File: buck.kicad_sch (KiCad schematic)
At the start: 23 parts, among them IC2 LV2862YDDCR, IC2 RT6285GSP

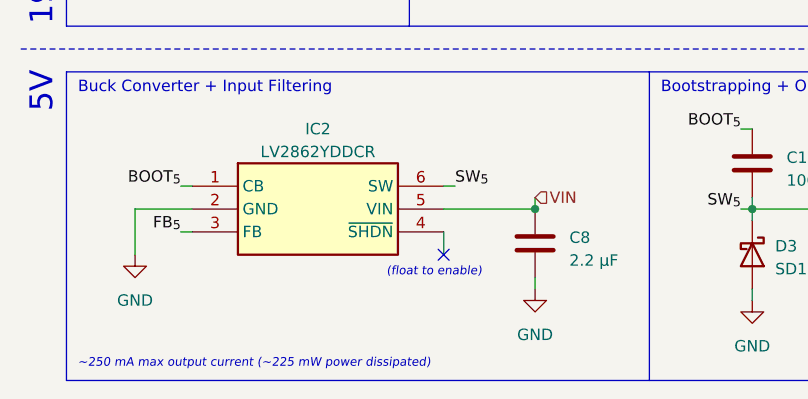
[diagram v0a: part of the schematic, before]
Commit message: Create new STEP files
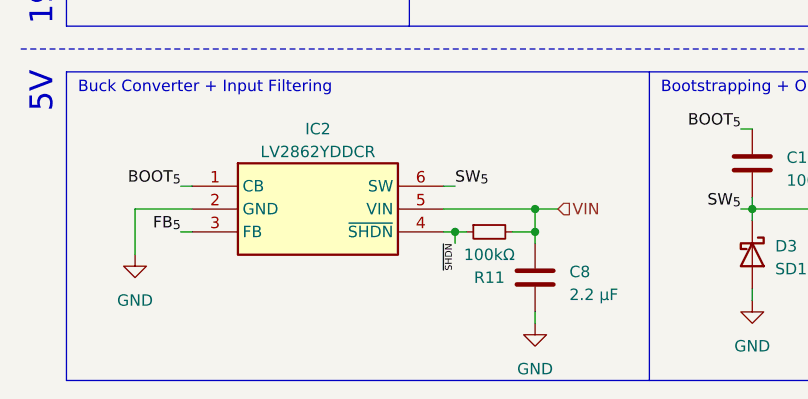
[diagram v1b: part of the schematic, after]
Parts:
- added R11: 100kΩ, Resistor_SMD:R_0603_1608Metric_Pad0.98x0.95mm_HandSolder, symbol Device:R_Small
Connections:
- net VIN: now also R11.2
- net ~{SHDN}: now reaches IC2.4 (~{SHDN})
- net ~{SHDN}: now also R11.1
- no-connect marks 4 -> 3
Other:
- note removed: "(float to enable)"
- note removed: "~250 mA max output current (~225 mW power dissipated)"
- moved on the sheet: C8
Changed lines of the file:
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@@
     (company "UT RoboMasters")
   )
+  (junction (at 91.44 133.35) (diameter 0) (color 0 0 0 0)
+  )
   (junction (at 100.33 130.81) (diameter 0) (color 0 0 0 0)
   )
@@
   (junction (at 135.89 57.15) (diameter 0) (color 0 0 0 0)
   )
+  (junction (at 100.33 133.35) (diameter 0) (color 0 0 0 0)
+  )
   (junction (at 97.79 60.96) (diameter 0) (color 0 0 0 0)
   )
@@
   )
   (no_connect (at 170.18 69.85))
-  (no_connect (at 90.17 135.89))
   (no_connect (at 200.66 74.93))
   (no_connect (at 170.18 72.39))
@@
     (stroke (width 0) (type default))
   )
-  (wire (pts (xy 90.17 135.89) (xy 90.17 133.35))
+  (wire (pts (xy 102.87 130.81) (xy 100.33 130.81))
     (stroke (width 0) (type default))
   )
@@
   )
   (wire (pts (xy 124.46 129.54) (xy 124.46 130.81))
+    (stroke (width 0) (type default))
+  )
+  (wire (pts (xy 91.44 134.62) (xy 91.44 133.35))
     (stroke (width 0) (type default))
   )
@@
     (stroke (width 0) (type dash))
   )
-  (wire (pts (xy 100.33 138.43) (xy 100.33 139.7))
+  (wire (pts (xy 100.33 142.24) (xy 100.33 143.51))
     (stroke (width 0) (type default))
   )
@@
     (stroke (width 0) (type default))
   )
+  (wire (pts (xy 97.79 133.35) (xy 100.33 133.35))
+    (stroke (width 0) (type default))
+  )
+  (wire (pts (xy 100.33 133.35) (xy 100.33 130.81))
+    (stroke (width 0) (type default))
+  )
   (polyline (pts (xy 86.36 78.74) (xy 156.21 78.74))
     (stroke (width 0) (type default))
   )
+  (wire (pts (xy 90.17 133.35) (xy 91.44 133.35))
+    (stroke (width 0) (type default))
+  )
   (wire (pts (xy 133.35 97.79) (xy 133.35 99.06))
     (stroke (width 0) (type default))
@@
     (stroke (width 0) (type default))
   )
-  (wire (pts (xy 100.33 129.54) (xy 100.33 130.81))
+  (wire (pts (xy 100.33 134.62) (xy 100.33 133.35))
     (stroke (width 0) (type default))
   )
@@
     (stroke (width 0) (type default))
   )
+  (wire (pts (xy 91.44 133.35) (xy 92.71 133.35))
+    (stroke (width 0) (type default))
+  )
   (wire (pts (xy 123.19 121.92) (xy 124.46 121.92))
     (stroke (width 0) (type default))
@@
   (wire (pts (xy 144.78 130.81) (xy 146.05 130.81))
     (stroke (width 0) (type default))
-  )
-  (text "(float to enable)" (at 83.82 138.43 0)
-    (effects (font (size 0.96 0.96) italic) (justify left bottom))
   )
   (text "Buck converter controller" (at 158.75 49.53 0)
@@
     (effects (font (size 1.27 1.27)) (justify left bottom))
   )
-  (text "~250 mA max output current (~225 mW power dissipated)"
-    (at 49.53 148.59 0)
-    (effects (font (size 0.96 0.96) italic) (justify left bottom))
-  )
   (label "BOOT_{5}" (at 123.19 121.92 180) (fields_autoplaced)
     (effects (font (size 1.27 1.27)) (justify right bottom))
   )
+  (label "~{SHDN}" (at 91.44 134.62 270) (fields_autoplaced)
+    (effects (font (size 0.762 0.762)) (justify right bottom))
+  )
   (label "BOOT_{19}" (at 168.91 67.31 180) (fields_autoplaced)
     (effects (font (size 1.27 1.27)) (justify right bottom))
@@
     (effects (font (size 1.27 1.27)) (justify left))
   )
-  (hierarchical_label "VIN" (shape input) (at 100.33 129.54 0) (fields_autoplaced)
+  (hierarchical_label "VIN" (shape input) (at 102.87 130.81 0) (fields_autoplaced)
     (effects (font (size 1.27 1.27)) (justify left))
   )
@@
     )
   )
-  (symbol (lib_id "Device:C") (at 100.33 134.62 0) (unit 1)
+  (symbol (lib_id "Device:C") (at 100.33 138.43 0) (unit 1)
     (in_bom yes) (on_board yes) (dnp no)
-    (property "Reference" "C8" (at 104.14 133.985 0)
-      (effects (font (size 1.27 1.27)) (justify left))
-    )
-    (property "Value" "2.2 μF" (at 104.14 136.525 0)
-      (effects (font (size 1.27 1.27)) (justify left))
-    )
-    (property "Footprint" "Capacitor_SMD:C_0603_1608Metric_Pad1.08x0.95mm_HandSolder" (at 101.2952 138.43 0)
-      (effects (font (size 1.27 1.27)) hide)
-    )
-    (property "Datasheet" "https://www.mouser.com/datasheet/2/585/MLCC-1837944.pdf" (at 100.33 134.62 0)
+    (property "Reference" "C8" (at 104.14 137.795 0)
+      (effects (font (size 1.27 1.27)) (justify left))
+    )
+    (property "Value" "2.2 μF" (at 104.14 140.335 0)
+      (effects (font (size 1.27 1.27)) (justify left))
+    )
+    (property "Footprint" "Capacitor_SMD:C_0603_1608Metric_Pad1.08x0.95mm_HandSolder" (at 101.2952 142.24 0)
+      (effects (font (size 1.27 1.27)) hide)
+    )
+    (property "Datasheet" "https://www.mouser.com/datasheet/2/585/MLCC-1837944.pdf" (at 100.33 138.43 0)
       (effects (font (size 1.27 1.27)) hide)
     )
@@
     )
   )
-  (symbol (lib_id "power:GND") (at 100.33 139.7 0) (unit 1)
-    (in_bom yes) (on_board yes) (dnp no) (fields_autoplaced)
-    (property "Reference" "#PWR035" (at 100.33 146.05 0)
-      (effects (font (size 1.27 1.27)) hide)
-    )
-    (property "Value" "GND" (at 100.33 144.78 0)
-      (effects (font (size 1.27 1.27)))
-    )
-    (property "Footprint" "" (at 100.33 139.7 0)
-      (effects (font (size 1.27 1.27)) hide)
-    )
-    (property "Datasheet" "" (at 100.33 139.7 0)
-      (effects (font (size 1.27 1.27)) hide)
-    )
+  (symbol (lib_id "Device:R_Small") (at 95.25 133.35 90) (mirror x) (unit 1)
+    (in_bom yes) (on_board yes) (dnp no)
+    (property "Reference" "R11" (at 95.25 138.43 90)
+      (effects (font (size 1.27 1.27)))
+    )
+    (property "Value" "100kΩ" (at 95.25 135.89 90)
+      (effects (font (size 1.27 1.27)))
+    )
+    (property "Footprint" "Resistor_SMD:R_0603_1608Metric_Pad0.98x0.95mm_HandSolder" (at 95.25 133.35 0)
+      (effects (font (size 1.27 1.27)) hide)
+    )
+    (property "Datasheet" "~" (at 95.25 133.35 0)
+      (effects (font (size 1.27 1.27)) hide)
+    )
+    (pin "1")
+    (pin "2")
+    (instances
+      (project "Chassis"
+        (path "/d5f28ba3-2393-441a-9a3a-5aa9d797472a/632f64e1-f4ac-4fce-8dc1-2a6086852be0"
+          (reference "R11") (unit 1)
+        )
+      )
+    )
+  )
+  (symbol (lib_id "power:GND") (at 100.33 143.51 0) (unit 1)
+    (in_bom yes) (on_board yes) (dnp no) (fields_autoplaced)
+    (property "Reference" "#PWR035" (at 100.33 149.86 0)
+      (effects (font (size 1.27 1.27)) hide)
+    )
+    (property "Value" "GND" (at 100.33 148.59 0)
+      (effects (font (size 1.27 1.27)))
+    )
+    (property "Footprint" "" (at 100.33 143.51 0)
+      (effects (font (size 1.27 1.27)) hide)
+    )
+    (property "Datasheet" "" (at 100.33 143.51 0)
+      (effects (font (size 1.27 1.27)) hide)
+    )

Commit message: Update libraries & changed footprints
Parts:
- D4: footprint Robomaster_ICs:SODFL5336X110N -> Robomaster_Passives:SODFL5336X110N
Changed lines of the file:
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@@
       (effects (font (size 1.27 1.27)) (justify left))
     )
-    (property "Footprint" "Robomaster_ICs:SODFL5336X110N" (at 107.95 95.25 0)
+    (property "Footprint" "Robomaster_Passives:SODFL5336X110N" (at 107.95 95.25 0)
       (effects (font (size 1.27 1.27)) hide)
     )

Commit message: BOMs away
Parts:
- C1, C12: Mouser Part Number (none) -> 603-CC0603JRX70BB103
- C11: Mouser Part Number (none) -> 187-CL10B104KB85PNL
- C3: Mouser Part Number (none) -> 187-CL10C820JB81PNC
- C5, C6: Mouser Part Number (none) -> 187-CL21A226MAYNNNE
- C7, C8: Mouser Part Number (none) -> 81-GRM188R6YA475KE5D
- C8: Mouser Part Number (none) -> 81-GRM188R6YA225KA2D
- R11, R3: Mouser Part Number (none) -> 791-RMC1/16K1003FTP
- R4: Mouser Part Number (none) -> 603-AC0603FR-076K8L
- R8: Mouser Part Number (none) -> 603-RC0603FR-0756RL
- R9: Mouser Part Number (none) -> 791-RMC16K103FTP
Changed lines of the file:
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@@
+      (effects (font (size 1.27 1.27)) hide)
+    )
+    (property "Mouser Part Number" "81-GRM188R6YA475KE5D" (at 142.24 60.96 0)
       (effects (font (size 1.27 1.27)) hide)
     )
@@
       (effects (font (size 1.27 1.27)) hide)
     )
+    (property "Mouser Part Number" "187-CL10C820JB81PNC" (at 110.49 55.88 0)
+      (effects (font (size 1.27 1.27)) hide)
+    )
     (pin "1")
     (pin "2")
@@
     )
     (property "Datasheet" "~" (at 97.79 66.04 0)
+      (effects (font (size 1.27 1.27)) hide)
+    )
+    (property "Mouser Part Number" "603-AC0603FR-076K8L" (at 97.79 66.04 0)
       (effects (font (size 1.27 1.27)) hide)
     )
@@
       (effects (font (size 1.27 1.27)) hide)
     )
+    (property "Mouser Part Number" "603-CC0603JRX70BB103" (at 71.12 83.82 0)
+      (effects (font (size 1.27 1.27)) hide)
+    )
     (pin "1")
     (pin "2")
@@
     )
     (property "Datasheet" "~" (at 172.72 127 0)
+      (effects (font (size 1.27 1.27)) hide)
+    )
+    (property "Mouser Part Number" "603-RC0603FR-0756RL" (at 172.72 127 0)
       (effects (font (size 1.27 1.27)) hide)
     )
@@
       (effects (font (size 1.27 1.27)) hide)
     )
+    (property "Mouser Part Number" "81-GRM188R6YA475KE5D" (at 135.89 60.96 0)
+      (effects (font (size 1.27 1.27)) hide)
+    )
     (pin "1")
     (pin "2")
@@
     )
     (property "Datasheet" "~" (at 144.78 135.89 0)
+      (effects (font (size 1.27 1.27)) hide)
+    )
+    (property "Mouser Part Number" "603-CC0603JRX70BB103" (at 144.78 135.89 0)
       (effects (font (size 1.27 1.27)) hide)
     )
@@
       (effects (font (size 1.27 1.27)) hide)
     )
+    (property "Mouser Part Number" "187-CL21A226MAYNNNE" (at 127 93.98 0)
+      (effects (font (size 1.27 1.27)) hide)
+    )
     (pin "1")
     (pin "2")
@@
       (effects (font (size 1.27 1.27)) hide)
     )
+    (property "Mouser Part Number" "187-CL21A226MAYNNNE" (at 133.35 93.98 0)
+      (effects (font (size 1.27 1.27)) hide)
+    )
     (pin "1")
     (pin "2")
@@
       (effects (font (size 1.27 1.27)) hide)
     )
+    (property "Mouser Part Number" "791-RMC1/16K1003FTP" (at 97.79 55.88 0)
+      (effects (font (size 1.27 1.27)) hide)
+    )
     (pin "1")
     (pin "2")
@@
     )
     (property "Datasheet" "~" (at 172.72 137.16 0)
+      (effects (font (size 1.27 1.27)) hide)
+    )
+    (property "Mouser Part Number" "791-RMC16K103FTP" (at 172.72 137.16 0)
       (effects (font (size 1.27 1.27)) hide)
     )
@@
       (effects (font (size 1.27 1.27)) hide)
     )
+    (property "Mouser Part Number" "81-GRM188R6YA225KA2D" (at 100.33 138.43 0)
+      (effects (font (size 1.27 1.27)) hide)
+    )
     (pin "1")
     (pin "2")
@@
       (effects (font (size 1.27 1.27)) hide)
     )
+    (property "Mouser Part Number" "187-CL10B104KB85PNL" (at 124.46 125.73 0)
+      (effects (font (size 1.27 1.27)) hide)
+    )
     (pin "1")
     (pin "2")
@@
       (effects (font (size 1.27 1.27)) hide)
     )
+    (property "Mouser Part Number" "791-RMC1/16K1003FTP" (at 95.25 133.35 0)
+      (effects (font (size 1.27 1.27)) hide)
+    )
